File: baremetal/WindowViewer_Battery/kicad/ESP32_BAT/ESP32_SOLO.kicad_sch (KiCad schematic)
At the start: 24 parts, among them J1 Conn_01x04_Male, J2 Conn_01x02_Male, U1 ESP32-S2-WROVER

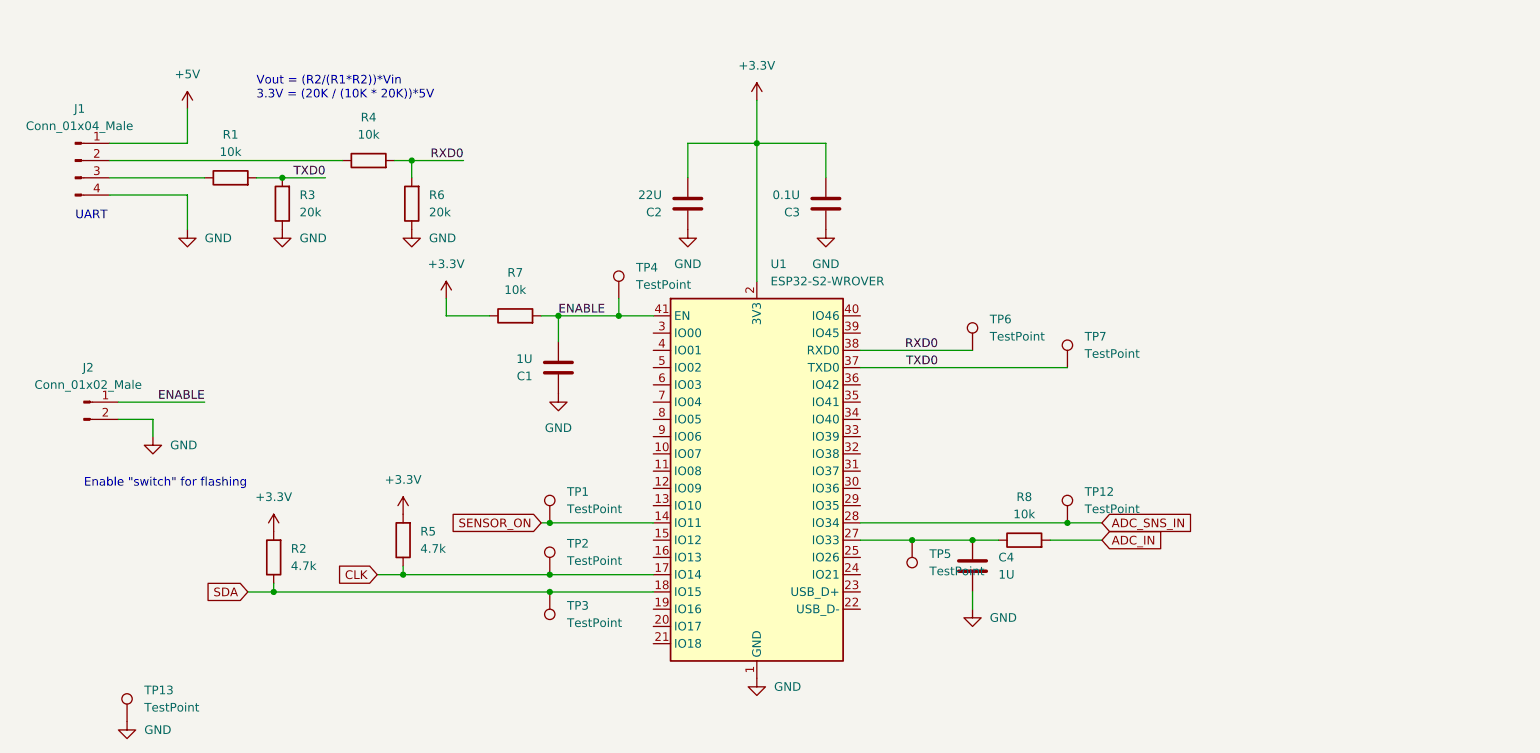
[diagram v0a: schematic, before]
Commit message: watersensor 0.1
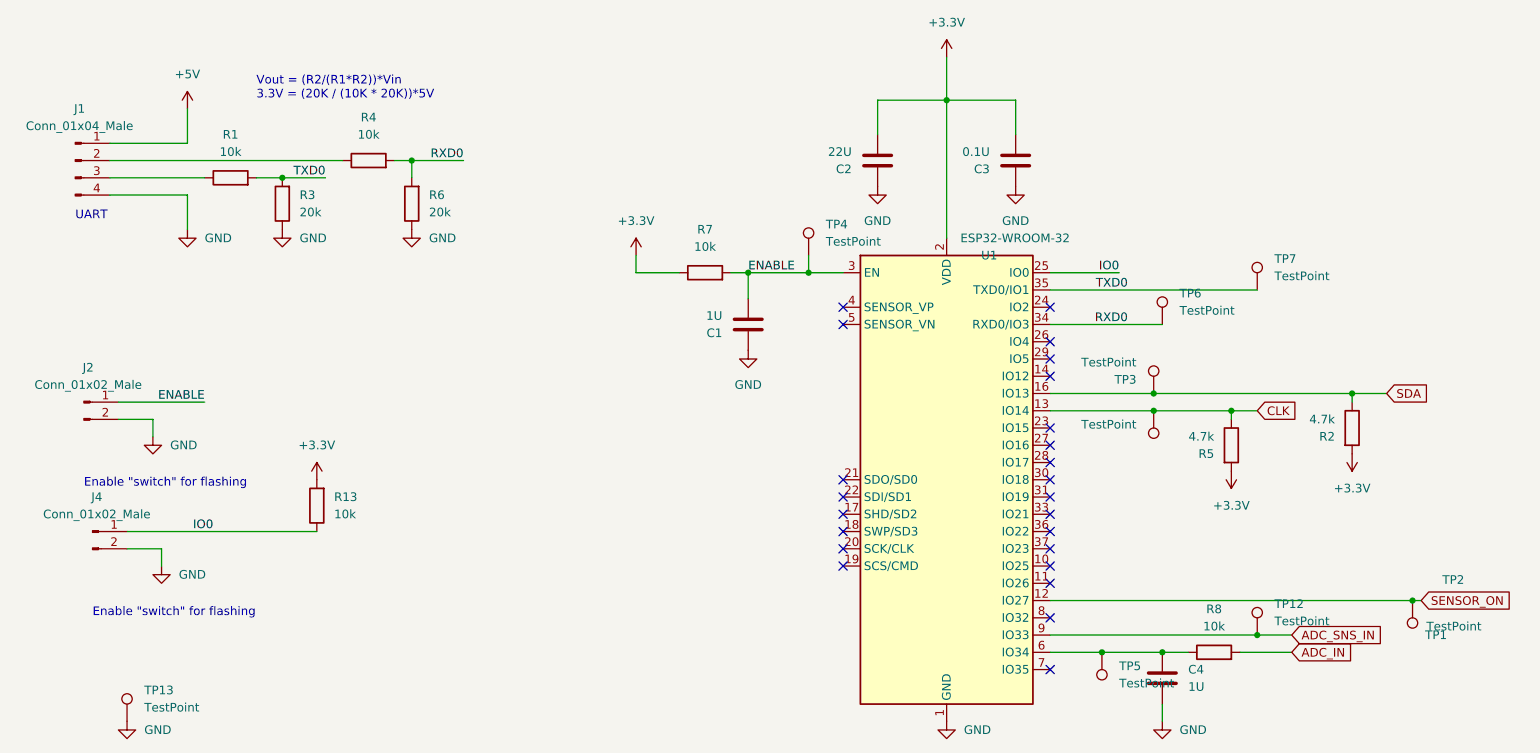
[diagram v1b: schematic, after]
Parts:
- removed U1: ESP32-S2-WROVER, RF_Module:ESP32-S2-WROVER, symbol RF_Module:ESP32-S2-WROVER
- added J4: Conn_01x02_Male, Connector_PinHeader_2.54mm:PinHeader_1x02_P2.54mm_Vertical, symbol Connector:Conn_01x02_Male
- added R13: 10k, Resistor_SMD:R_1206_3216Metric_Pad1.30x1.75mm_HandSolder, symbol Device:R
- added U1: ESP32-WROOM-32, RF_Module:ESP32-WROOM-32, symbol RF_Module:ESP32-WROOM-32
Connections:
- net +3V3: now also R13.2, U1.2 (VDD)
- net ADC_SNS_IN: now also U1.9 (IO33)
- net CLK: now also U1.13 (IO14)
- net ENABLE: now also U1.3 (EN)
- net GND: now also J4.2 (Pin_2), U1.1 (GND), U1.15 (GND), U1.38 (GND), U1.39 (GND)
- net RXD0: now also U1.34 (RXD0/IO3)
- net SDA: now also U1.16 (IO13)
- net SENSOR_ON: now also U1.12 (IO27)
- net TXD0: now also U1.35 (TXD0/IO1)
- net at C4.1, R8.1, TP5.1: now also U1.6 (IO34)
- new net IO0: J4.1 (Pin_1), R13.1, U1.25 (IO0)
- no-connect marks 0 -> 24
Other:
- moved on the sheet: C1, C2, C3, C4, R2, R5, R7, R8, TP1, TP12, TP2, TP3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
